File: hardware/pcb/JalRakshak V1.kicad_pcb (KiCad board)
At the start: 2 copper layers, 130 x 105.5 mm, 12 parts, among them U1 ESP32-WROOM-32

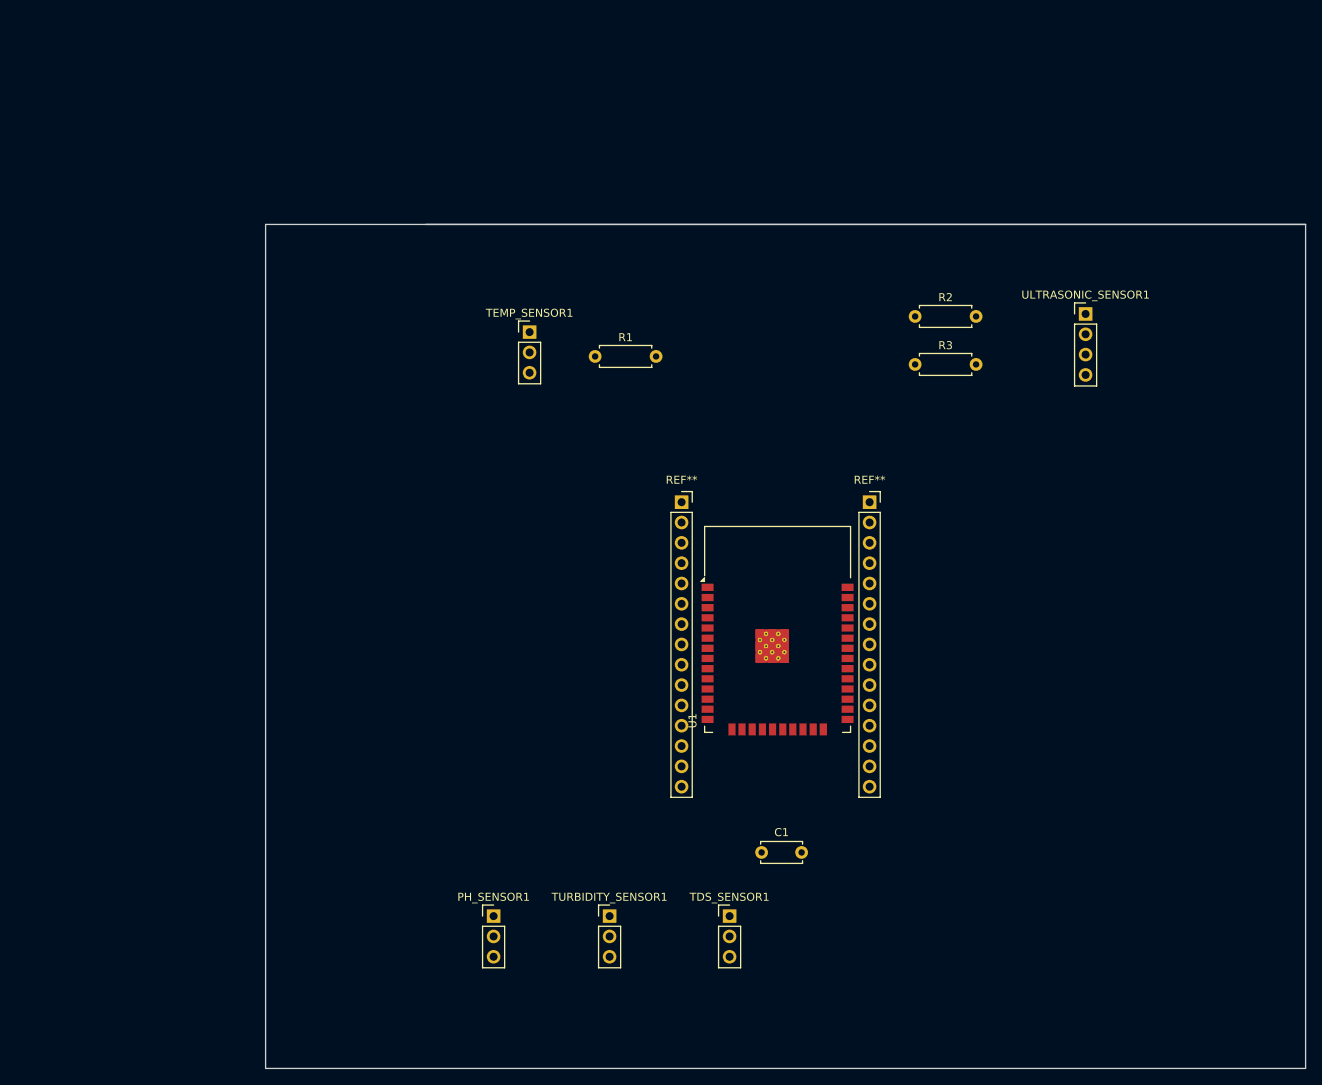
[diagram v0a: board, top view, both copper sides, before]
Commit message: Add files via upload
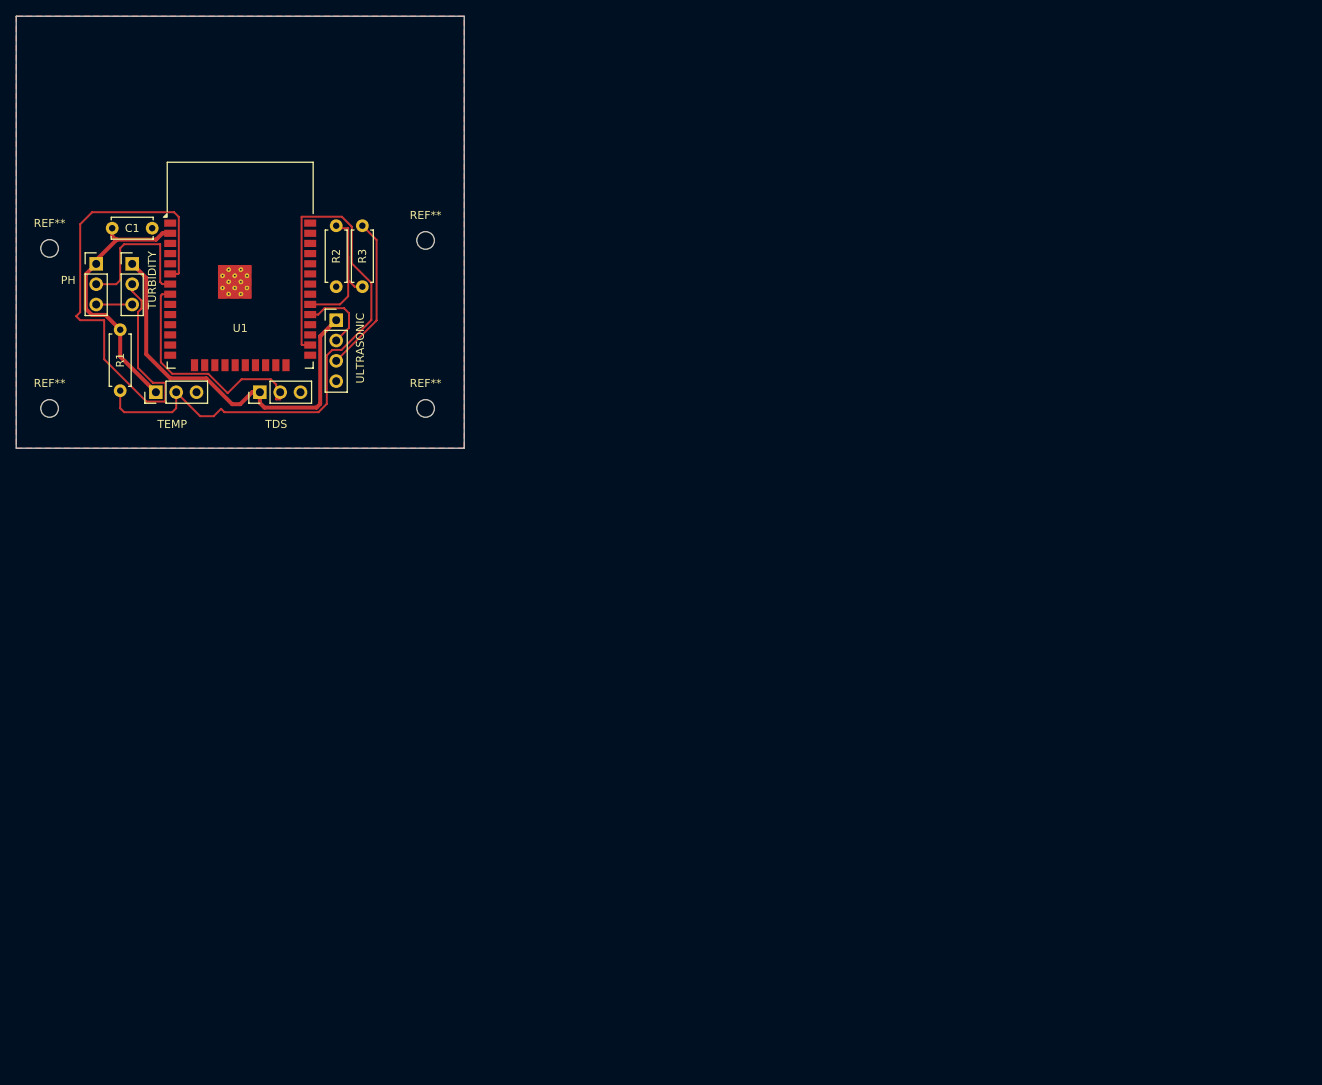
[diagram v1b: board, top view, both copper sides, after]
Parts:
- removed the REF** at (122.0, 74.7)
- removed the REF** at (145.5, 74.7)
- added REF**: MountingHole_2.2mm_M2, MountingHole:MountingHole_2.2mm_M2, F.Cu at (90.0, 63.0)
- added REF**: MountingHole_2.2mm_M2, MountingHole:MountingHole_2.2mm_M2, F.Cu at (43.0, 63.0)
- added REF**: MountingHole_2.2mm_M2, MountingHole:MountingHole_2.2mm_M2, F.Cu at (43.0, 43.0)
- added REF**: MountingHole_2.2mm_M2, MountingHole:MountingHole_2.2mm_M2, F.Cu at (90.0, 42.0)
- moved C1 112.6 mm to (50.8, 40.5)
- moved TURBIDITY 101.0 mm to (53.3, 44.9)
- moved PH 95.5 mm to (48.8, 44.9)
- moved ULTRASONIC 93.7 mm to (78.8, 52.0)
- moved TDS 88.0 mm to (69.3, 61.0), turned to 90 degrees
- moved U1 81.2 mm to (66.8, 48.1)
- moved R2 72.5 mm to (78.8, 47.8), turned to 90 degrees
- moved R3 69.8 mm to (82.1, 47.8), turned to 90 degrees
- moved R1 59.5 mm to (51.8, 60.8), turned to 90 degrees
- moved TEMP 47.3 mm to (56.3, 61.0), turned to 90 degrees
- renumbered PH_SENSOR1 to PH, TDS_SENSOR1 to TDS, TEMP_SENSOR1 to TEMP, TURBIDITY_SENSOR1 to TURBIDITY, ULTRASONIC_SENSOR1 to ULTRASONIC
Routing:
- net /TEMP_DATA: track 0.00 -> 83.2 mm
- net /TURBIDITY_SIGNAL: track 0.00 -> 69.1 mm
- net /+5V: track 0.00 -> 50.0 mm
- net +3.3V: track 0.00 -> 34.1 mm
- net /TDS_SIGNAL: track 0.00 -> 29.9 mm
- net /ULTRA_ECHO: track 0.00 -> 20.9 mm
- net /ULTRA_ECHO_RAW: track 0.00 -> 19.7 mm
- net /PH_SIGNAL: track 0.00 -> 18.5 mm
- net /ULTRA_TRIG: track 0.00 -> 9.51 mm
- net GND: track 0.00 -> 4.50 mm
- added copper zone on F.Cu, net GND
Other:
- board size 130 x 105.5 mm -> 56 x 54 mm
